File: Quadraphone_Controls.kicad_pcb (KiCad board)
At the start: 2 copper layers, 60 x 110 mm, 17 parts, among them J1 Conn_01x10_Female, J10 Pitch_In, J11 Mix_Out, J2 Conn_01x10_Female, J3 Conn_01x10_Female, J4 Conn_01x10_Female, J5 PWM_CV, J6 LFO_IN, J7 PWM_CV_In, J8 Synch_Signal_In, J9 Freq_Mod_In, SW1 Synch_Type, SW2 Output_Type

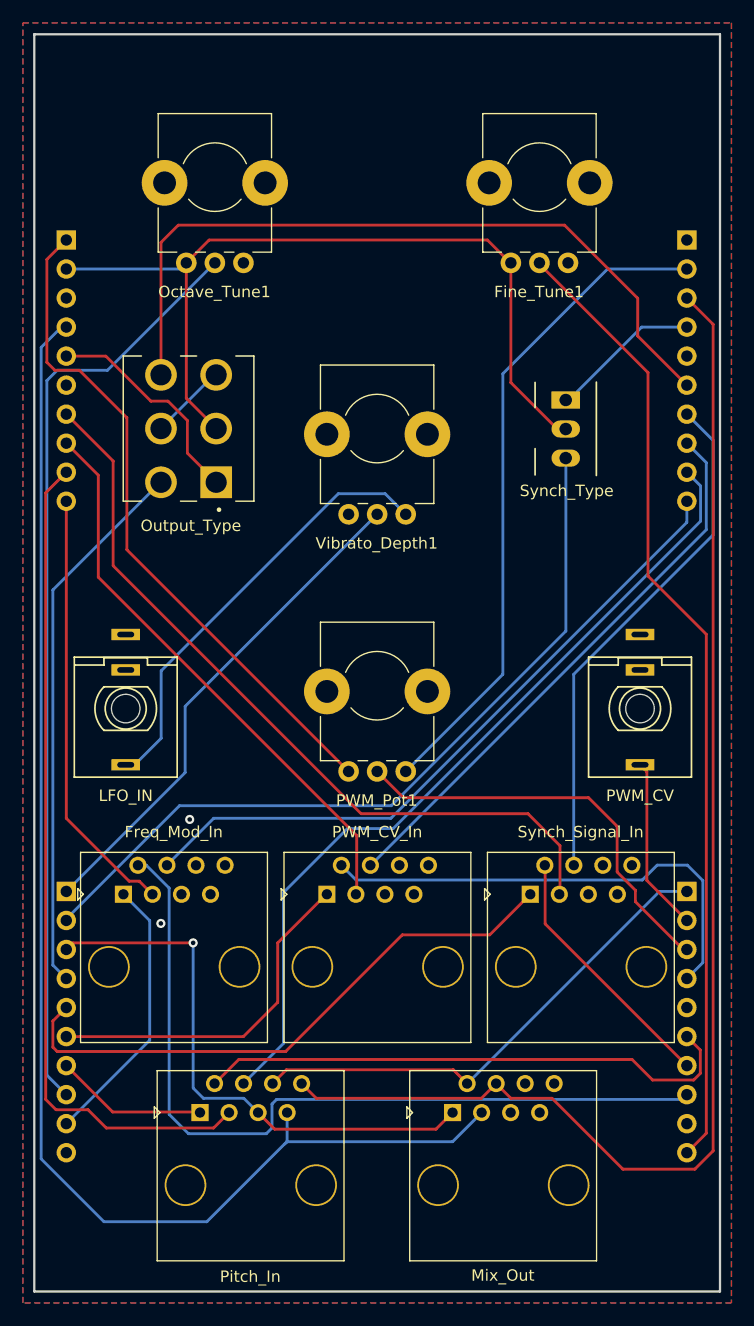
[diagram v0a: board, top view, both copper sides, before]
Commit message: First draft panel done
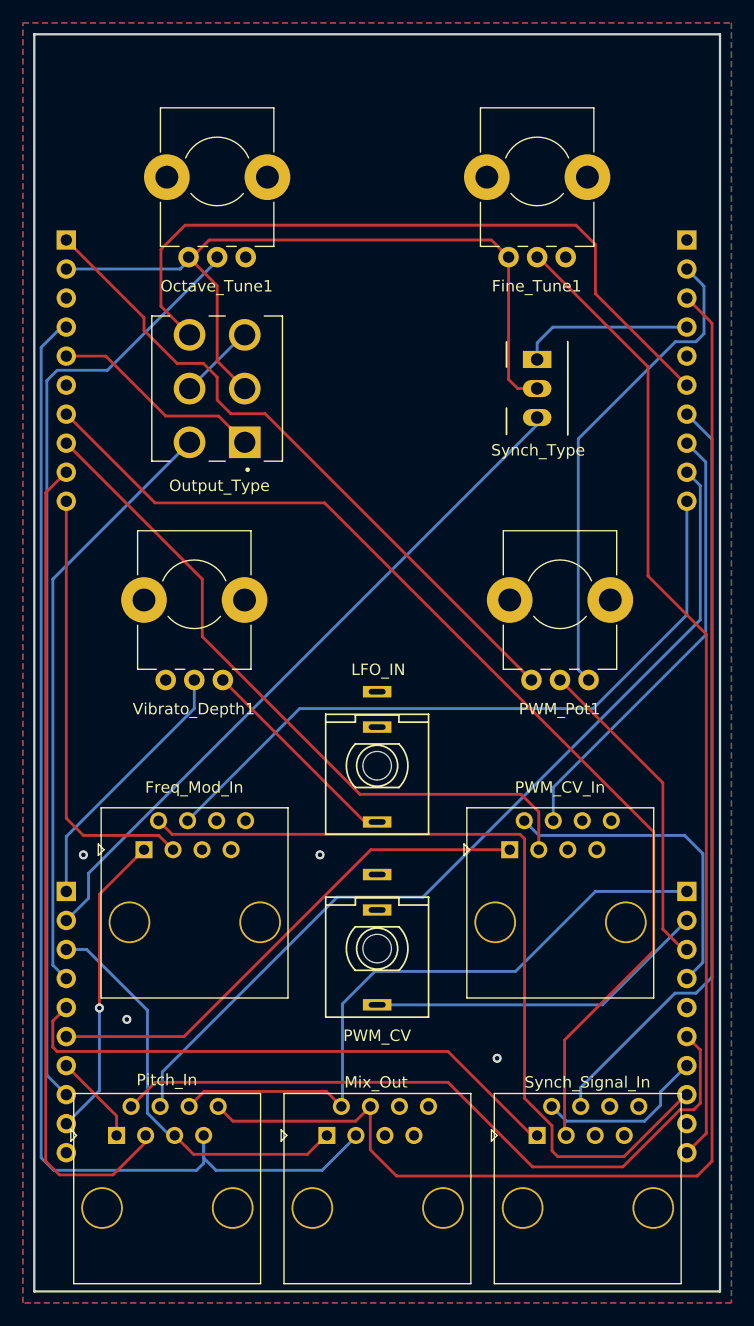
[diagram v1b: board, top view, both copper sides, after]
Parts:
- moved J5 31.1 mm to (80.0, 125.0)
- moved J6 22.6 mm to (80.0, 109.0)
- moved Vibrato_Depth1 21.6 mm to (64.0, 94.0)
- moved J8 21.1 mm to (98.4, 146.0)
- moved PWM_Pot1 17.9 mm to (96.0, 94.0)
- moved J7 16.5 mm to (96.0, 121.0)
- moved J11 11.2 mm to (80.0, 146.0)
- moved J10 7.57 mm to (61.6, 146.0)
- moved SW1 4.34 mm to (94.0, 73.5)
- moved SW2 4.30 mm to (66.0, 76.0)
- moved J9 4.30 mm to (64.0, 121.0)
- moved Fine_Tune1 0.54 mm to (94.0, 57.0)
- moved Octave_Tune1 0.54 mm to (66.0, 57.0)
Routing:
- net /SYNCH_SIGNAL2: track 68.5 -> 96.4 mm
- net /SYNCH_SIGNAL1: track 45.5 -> 67.3 mm
- net /LIN_FREQ_IN: track 44.3 -> 23.1 mm
- net /LFO_IN: track 38.5 -> 18.6 mm
- net -12V: track 58.2 -> 42.6 mm
- net /PWM_CV: track 15.3 -> 30.2 mm
- net /PWM_CV4: track 31.0 -> 45.6 mm
- net /V_PER_OCT3: track 48.2 -> 62.4 mm
- net /PWM_CV3: track 42.4 -> 28.3 mm
- net /MIX_OUT3: track 44.2 -> 57.6 mm
- net /MIX_OUT2: track 121.6 -> 108.3 mm
- net /MIX_OUT4: track 48.8 -> 36.2 mm, vias 1 -> 0
- net /PWM_CV2: track 50.2 -> 61.0 mm
- net /PWM_CV1: track 49.9 -> 39.2 mm
- net /MIX_OUT1: track 116.4 -> 126.0 mm
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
